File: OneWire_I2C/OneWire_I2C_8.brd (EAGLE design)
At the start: 22.2 x 28.2 mm, 14 parts, among them Q1 TP0602N3

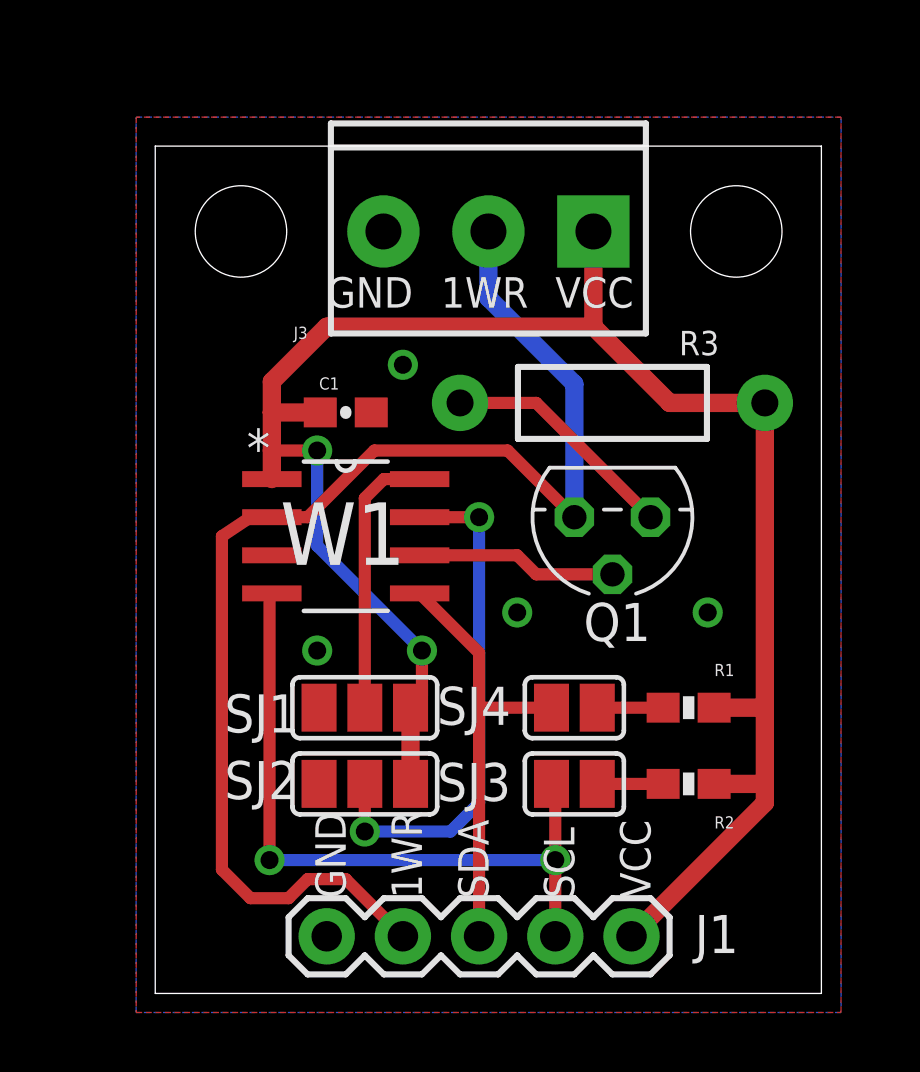
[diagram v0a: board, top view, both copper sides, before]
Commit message: Added Schematic and board for DS2482-800
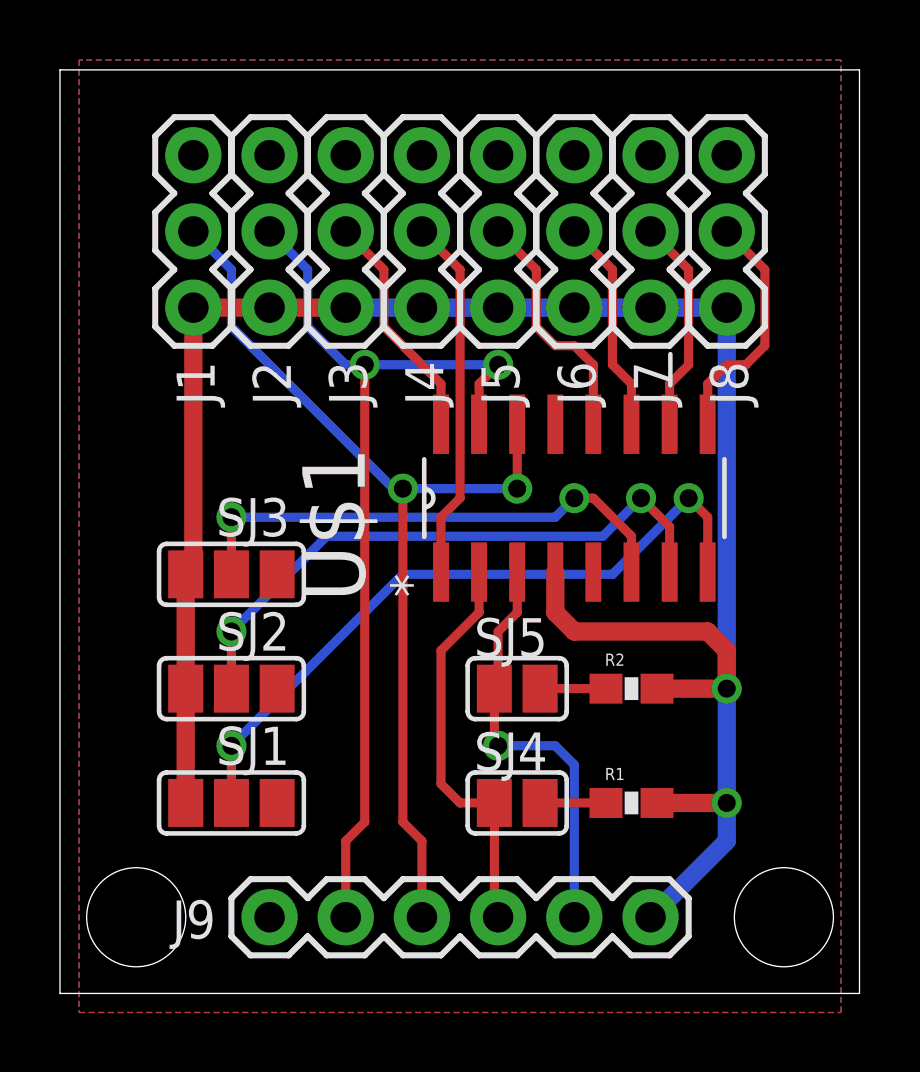
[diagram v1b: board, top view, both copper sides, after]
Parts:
- removed C1: (no value), SparkFun-Capacitors:0603-CAP
- removed Q1: TP0602N3, transistor-fet:TO-92
- removed R3: (no value), SparkFun-Resistors:AXIAL-0.4
- removed W1: DS2482-100, PuffinOneWIre:SOIC8
- added J2, J4, J5, J6, J7, J8: (no value), SparkFun-Connectors:1X03
- added J9: (no value), SparkFun-Connectors:1X06
- added SJ5: (no value), jumper:SJ
- added U$3: (no value), SparkFun-Electromechanical:STAND-OFF
- J1: device SparkFun-Connectors:1X05 -> SparkFun-Connectors:1X03
- J3: device SparkFun-Connectors:SCREWTERMINAL-3.5MM-3 -> SparkFun-Connectors:1X03
- R1, R2: device SparkFun-Resistors:0603-RES -> SparkFun-Passives:0603-RES
- SJ3: device jumper:SJ -> jumper:SJ_2
- U$1: value (none) -> DS2482-800; device SparkFun-Electromechanical:STAND-OFF-TIGHT -> Puffin:SOIC16
- U$2: device SparkFun-Electromechanical:STAND-OFF-TIGHT -> SparkFun-Electromechanical:STAND-OFF
- moved U$2 30.4 mm to (1.91, 2.54)
- moved J1 25.5 mm to (3.81, 22.9), turned to 90 degrees
- moved U$1 14.2 mm to (16.5, 16.5), turned to 90 degrees
- moved SJ3 13.4 mm to (5.08, 14.0)
- moved J3 8.64 mm to (8.89, 22.9), turned to 90 degrees
- moved SJ1 5.46 mm to (5.08, 6.35), turned to 0 degrees
- moved SJ2 5.46 mm to (5.08, 10.2), turned to 0 degrees
- moved R1 3.70 mm to (18.4, 6.35), turned to 0 degrees
- moved SJ4 3.70 mm to (14.6, 6.35), turned to 180 degrees
- moved R2 3.70 mm to (18.4, 10.2), turned to 0 degrees
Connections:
- removed net 1WR: J1.4, J3.2, Q1.3, W1.2
- removed net N$10: Q1.1, R3.P$1
- removed net N$3: R2.2, SJ3.2
- removed net N$4: R1.2, SJ4.2
- removed net PCTL: Q1.2, W1.6
- new net AD2: SJ3.2, U$1.6
- new net IO0: J1.2, J9.3, U$1.14
- new net IO1: J2.2, J9.2, U$1.15
- new net IO2: J3.2, U$1.16
- new net IO3: J4.2, U$1.1
- new net IO4: J5.2, U$1.12
- new net IO5: J6.2, U$1.11
- new net IO6: J7.2, U$1.10
- new net IO7: J8.2, U$1.9
- new net N$1: R1.1, SJ4.1
- new net N$2: R2.1, SJ5.1
- net AD0: now also U$1.8; no longer W1.8
- net AD1: now also U$1.7; no longer W1.7
- net GND: now also J1.3, J2.3, J4.3, J5.3, J6.3, J7.3, J8.3, J9.1, SJ3.3, U$1.13; no longer C1.2, J1.5, W1.3
- net SCL: now also J9.4, SJ4.2, U$1.2; no longer J1.2, SJ3.1, W1.4
- net SDA: now also J9.5, SJ5.2, U$1.3; no longer J1.3, SJ4.1, W1.5
- net VCC: now also J2.1, J4.1, J5.1, J6.1, J7.1, J8.1, J9.6, R1.2, R2.2, SJ3.1, U$1.4; no longer C1.1, R1.1, R2.1, R3.P$2, W1.1
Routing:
- net 1WR: track 42.4 -> 0.00 mm
- net IO0: track 0.00 -> 32.2 mm, vias 0 -> 2
- net IO1: track 0.00 -> 31.5 mm, vias 0 -> 2
- net AD2: track 0.00 -> 17.2 mm, vias 0 -> 2
- net AD0: track 9.08 -> 23.3 mm, vias 0 -> 2
- net IO3: track 0.00 -> 12.1 mm
- net SCL: track 23.7 -> 13.5 mm, vias 2 -> 0
- net IO7: track 0.00 -> 8.11 mm
- net IO4: track 0.00 -> 8.11 mm
- net N$10: track 7.93 -> 0.00 mm
- net IO2: track 0.00 -> 7.74 mm
- net IO6: track 0.00 -> 7.22 mm
- net IO5: track 0.00 -> 7.22 mm
- net PCTL: track 6.69 -> 0.00 mm
- net VCC: track 63.5 -> 69.3 mm
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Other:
- board size 22.2 x 28.2 mm -> 26.7 x 30.8 mm
- board text removed: "1WR"
- board text removed: "GND"
- board text removed: "SCL"
- board text removed: "SDA"
- board text removed: "VCC"
